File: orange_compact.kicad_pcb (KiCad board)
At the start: 6 copper layers, 50 x 45 mm, 171 parts, among them IC1 MCP25625-E_ML, IC2 MAX13487EESA+T, J1 SIM8060-6-0-14-00-A, J2 Conn_Coaxial, J3 Conn_Coaxial, J4 USB_B_Micro, J5 Conn_01x08_Pin, Q1 BC846A,215, Q2 BC846A,215, Q3 MMBT3904, Q4 MMBT3904, U1 NUP4202, U12 LM3671MF-3.3/NOPB, U13 LIS2DH12TR, U19 MX25R6435FZNIL0, U2 MDBT50Q-1M, U20 TPS566242DRLR, U3 FDMC86139P, U4 LM5012DDAR, U5 TXB0108DQSR, U6 EG915NEUAG-N06-SGNSA, U7 USBLC6-2SC6, Y2 16MHz

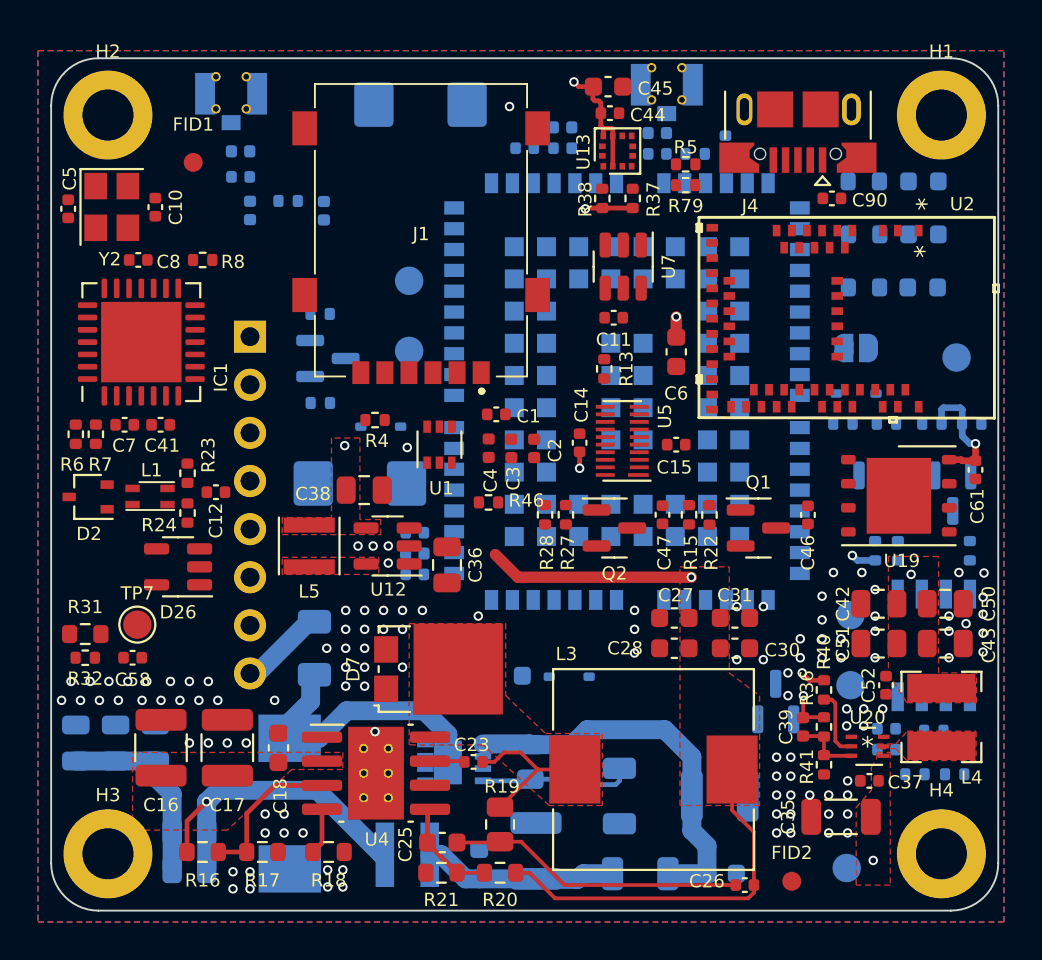
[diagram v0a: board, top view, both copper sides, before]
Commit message: saved 5/8
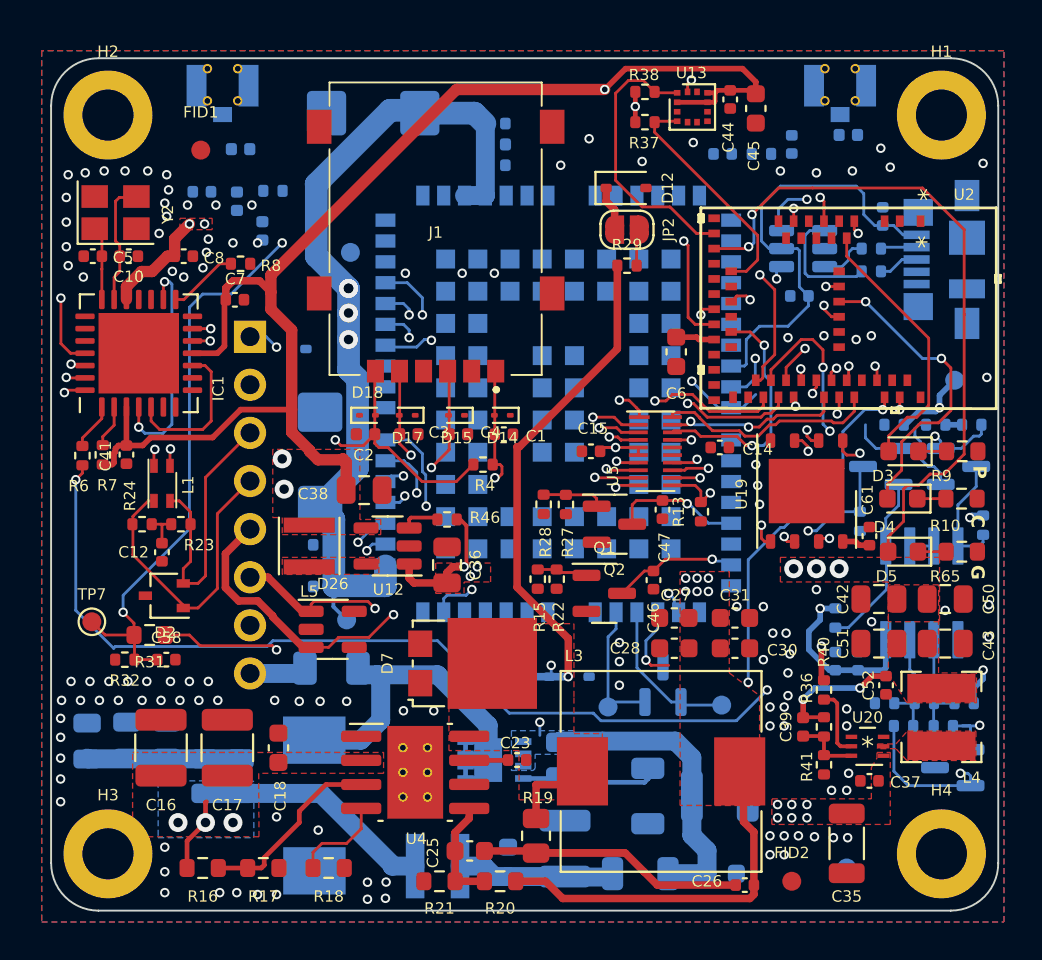
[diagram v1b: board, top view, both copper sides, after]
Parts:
- removed U1: NUP4202, Package_TO_SOT_SMD:SOT-363_SC-70-6
- added D14: ESD9C5.0ST5G, Diode_SMD:D_SOD-923, F.Cu at (137.2, 80.2)
- added D15: ESD9C5.0ST5G, Diode_SMD:D_SOD-923, F.Cu at (134.8, 80.2)
- added D17: ESD9C5.0ST5G, Diode_SMD:D_SOD-923, F.Cu at (132.2, 80.2)
- added D18: ESD9C5.0ST5G, Diode_SMD:D_SOD-923, F.Cu at (130.1, 80.2)
- C11, C90, R5, R79, U7: moved to B.Cu
- D12, D3, D4, D5, JP2, R10, R29, R65, R9: moved to F.Cu
- IC2: footprint max13487eesa:SOIC127P600X175-8N -> TC-ICs:SOIC127P600X175-8N
- J4: footprint Connector_USB:USB_Micro-B_XKB_U254-051T-4BH83-F1S -> Connector_USB:USB_Micro-B_Molex_47346-0001; moved to B.Cu
- TP2, TP3, TP4, TP5, TP6, TP7, TP8: footprint TestPoint:TestPoint_Pad_D1.5mm -> TestPoint:TestPoint_Pad_D1.0mm
- moved D16 39.4 mm to (161.0, 98.8), turned to 180 degrees
- moved R48 37.7 mm to (158.4, 96.6)
- moved R47 37.0 mm to (160.5, 96.6), turned to 180 degrees
- moved D12 16.3 mm to (143.8, 68.2)
- moved R9 15.2 mm to (161.5, 82.1), turned to 180 degrees
- moved R65 14.9 mm to (161.5, 87.4), turned to 180 degrees
- moved R10 14.9 mm to (161.5, 84.6), turned to 180 degrees
- moved TP8 14.6 mm to (129.0, 91.0)
- moved D3 14.3 mm to (158.4, 82.1), turned to 180 degrees
- moved R29 14.1 mm to (143.8, 72.3)
- moved D4 14.0 mm to (158.3, 84.6), turned to 180 degrees
- moved D5 14.0 mm to (158.4, 87.4), turned to 180 degrees
- moved TP3 13.7 mm to (142.8, 95.6)
- moved JP2 13.6 mm to (143.8, 70.4)
- moved R79 10.8 mm to (156.7, 72.6)
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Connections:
- C41 pad 1: 3V3_CAN -> 3V3_ALWAYS_ON
- C7 pad 1: 3V3_CAN -> 3V3_ALWAYS_ON
- C8 pad 2: NMEA_5V0 -> 5V0
- D2 pad 1: Net-(D2-A1) -> /CAN_500_L
- D2 pad 2: Net-(D2-A2) -> /CAN_500_H
- IC1 pad 11: NMEA_3V3 -> 3V3_ALWAYS_ON
- IC1 pad 12: Net-(D2-A1) -> Net-(IC1-CANL)
- IC1 pad 13: Net-(D2-A2) -> Net-(IC1-CANH)
- IC1 pad 19: NMEA_5V0 -> 5V0
- IC1 pad 3: 3V3_CAN -> 3V3_ALWAYS_ON
- L1 pad 1: Net-(D2-A2) -> Net-(IC1-CANH)
- L1 pad 4: Net-(D2-A1) -> Net-(IC1-CANL)
- R7 pad 2: 3V3_CAN -> 3V3_ALWAYS_ON
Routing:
- net /CAN_CS: track 0.00 -> 69.8 mm, vias 0 -> 3
- net 5V0: track 53.3 -> 122.0 mm, vias 2 -> 21
- net 1V8: track 0.00 -> 62.4 mm, vias 0 -> 3
- net /D-/B: track 0.00 -> 60.4 mm, vias 0 -> 2
- net /D+/A: track 0.00 -> 59.5 mm, vias 0 -> 1
- net /EBL: track 0.00 -> 59.2 mm, vias 0 -> 3
- net /SWDIO: track 0.00 -> 55.4 mm, vias 0 -> 3
- net /SWDCLK: track 0.00 -> 52.8 mm, vias 0 -> 2
- net /CAN_MISO: track 0.00 -> 51.3 mm, vias 0 -> 2
- net /CAN_MOSI: track 0.00 -> 47.7 mm, vias 0 -> 2
- net /CAN_SCK: track 0.00 -> 45.1 mm, vias 0 -> 2
- net /CAN_INT: track 0.00 -> 44.1 mm, vias 0 -> 2
- net /AUX_LED: track 0.00 -> 35.9 mm, vias 0 -> 2
- net /MODEM_RX_1V8: track 0.00 -> 34.3 mm, vias 0 -> 2
- net /MODEM_TX_1V8: track 0.00 -> 32.4 mm, vias 0 -> 2
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- added copper zone on B.Cu, net /EBL_60V
- added copper zone on In2.Cu, net 4V0
- added copper zone on In2.Cu, net 5V0
- added copper zone on B.Cu, net VIN
